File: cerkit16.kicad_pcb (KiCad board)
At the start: 2 copper layers, 79.5 x 79.5 mm, 35 parts, among them U1 ProMicro

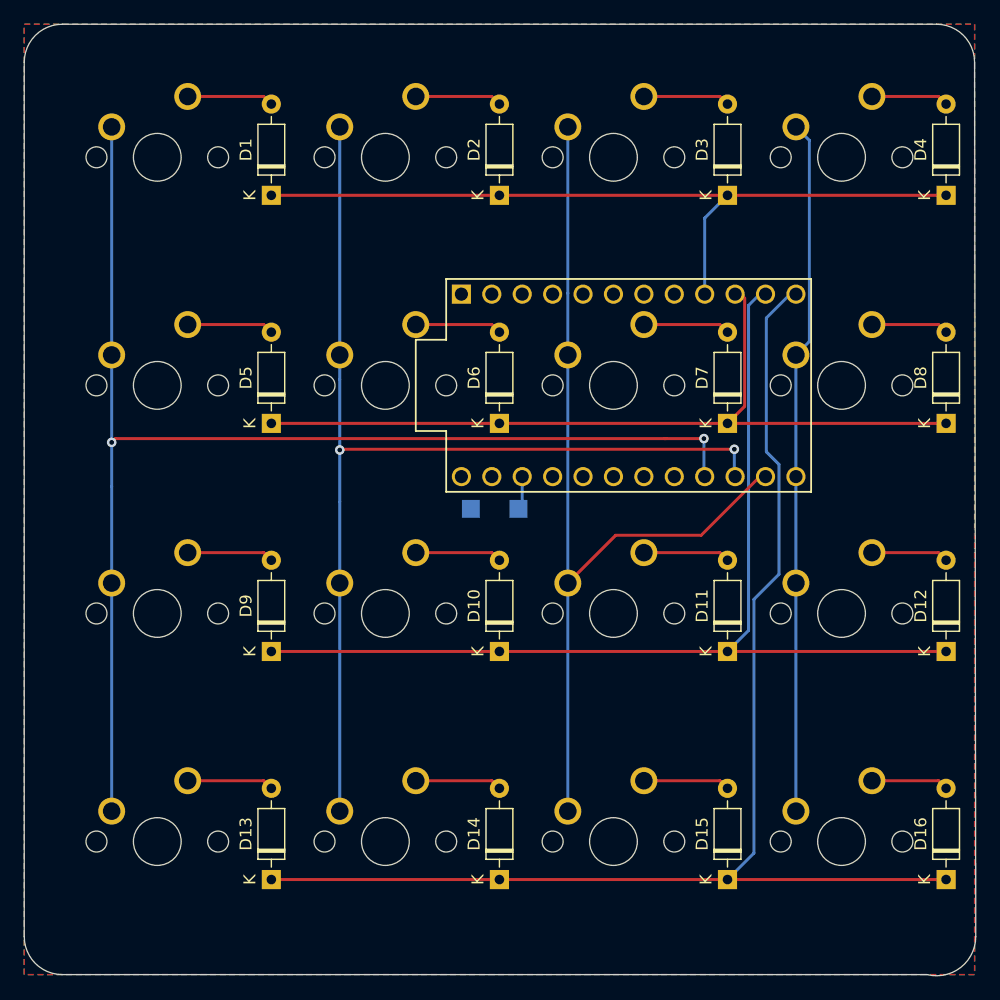
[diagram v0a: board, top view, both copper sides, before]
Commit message: added gerbers
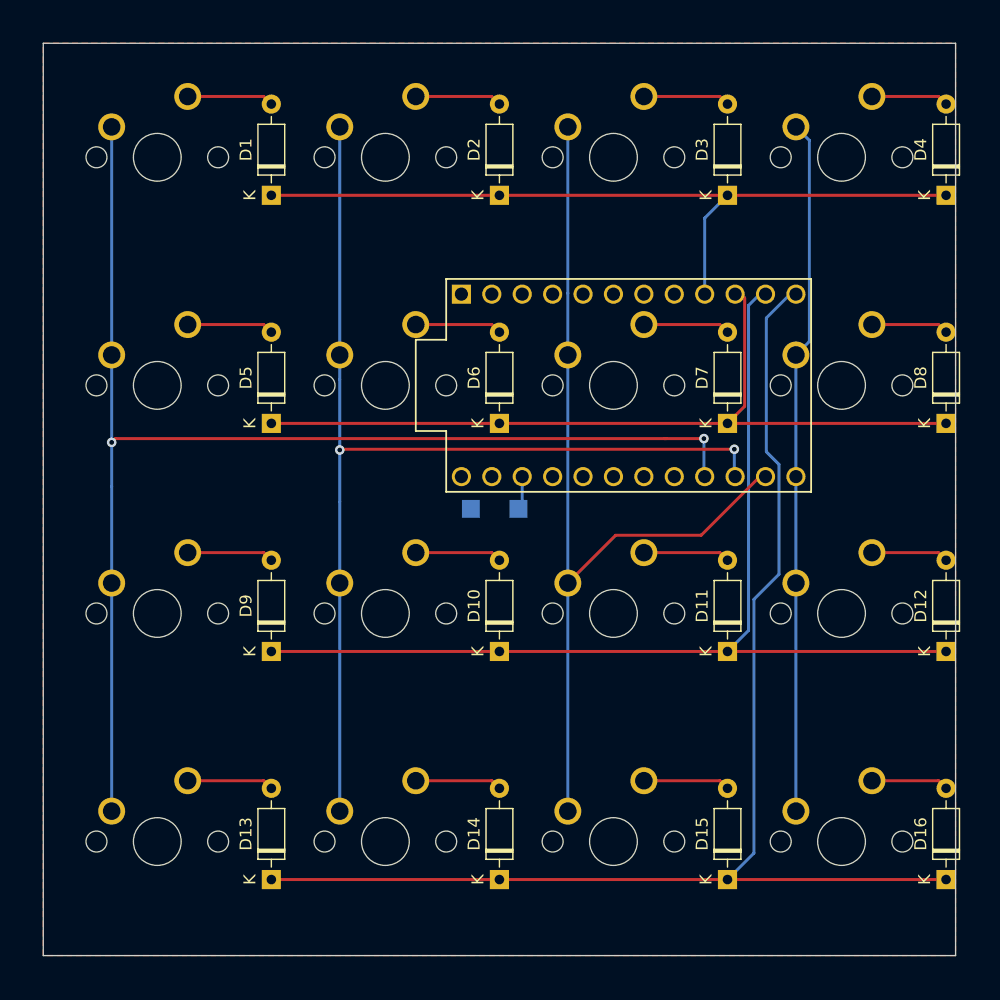
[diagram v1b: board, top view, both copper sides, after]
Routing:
- removed copper zone on B.Cu, net GND
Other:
- board size 79.5 x 79.5 mm -> 76.2 x 76.2 mm
